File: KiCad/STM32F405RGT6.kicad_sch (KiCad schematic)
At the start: 53 parts, among them J1 Conn_02x05_Odd_Even, J2 USB_C_Receptacle_USB2.0, SW1 TS-1187A, SW2 TS-1187A, U1 M24C02-RMN, U2 STM32F405RGTx, U3 AMS1117-3.3, U4 SRV05-4, Y1 16MHz

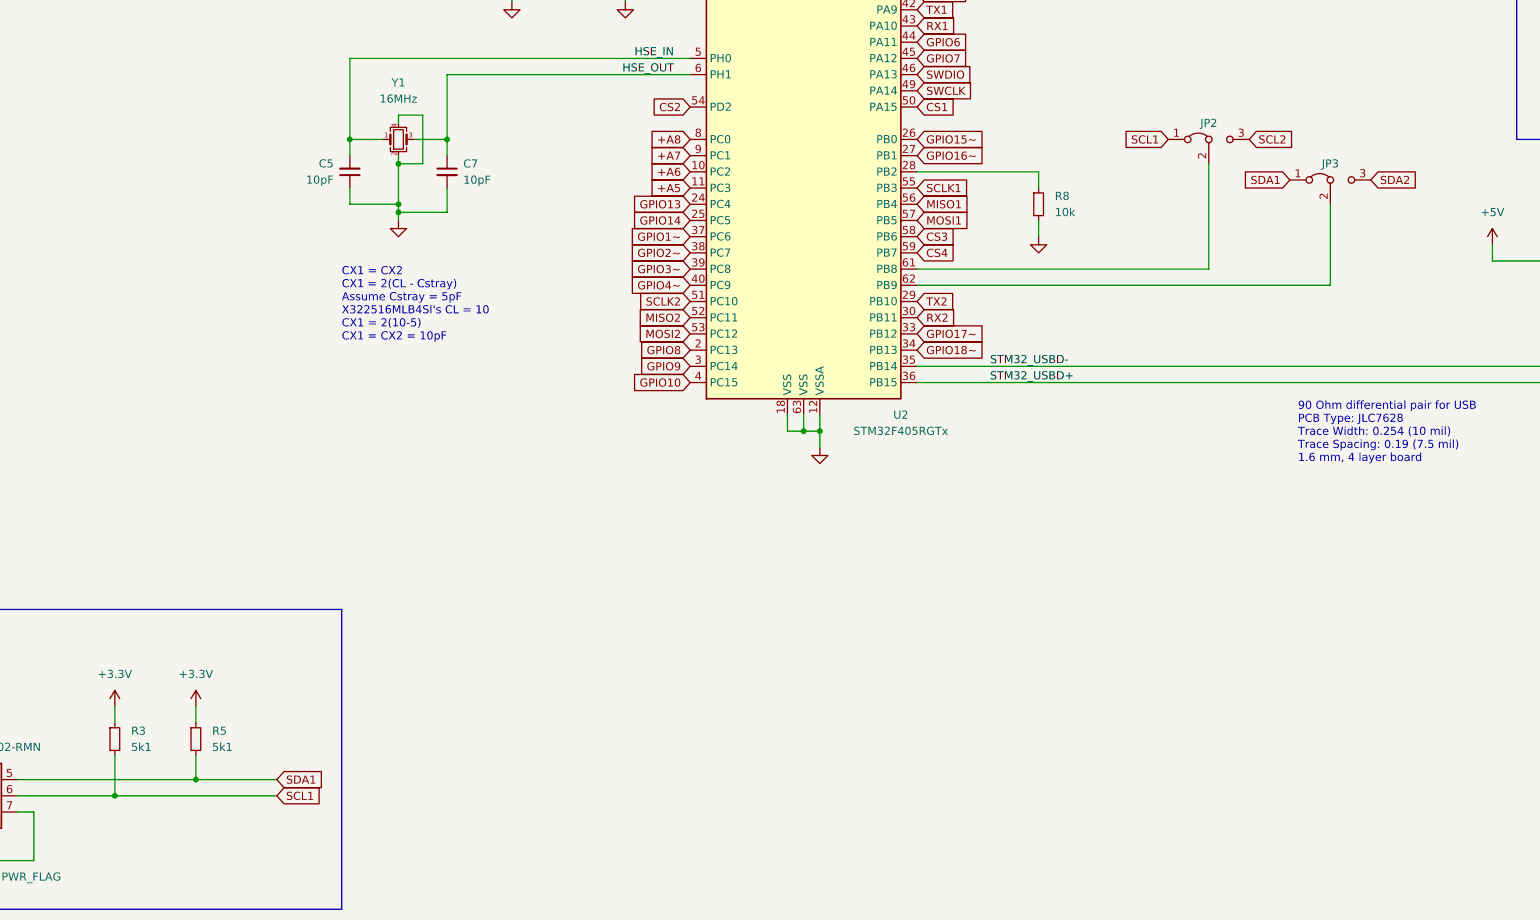
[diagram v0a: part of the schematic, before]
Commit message: Updated PCB and Schematic
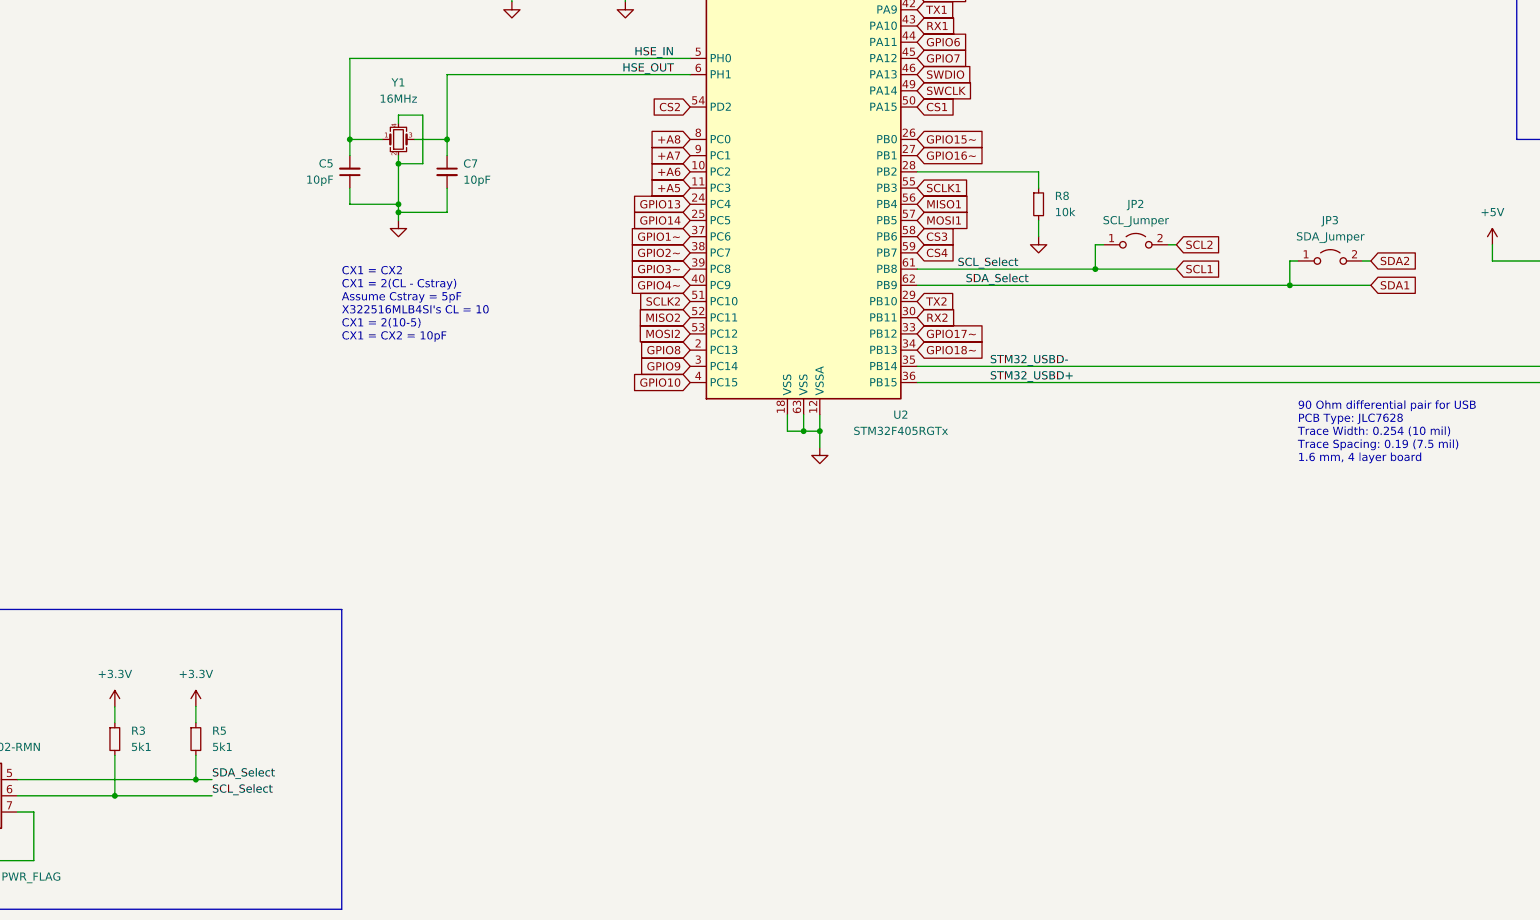
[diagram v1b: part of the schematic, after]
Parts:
- removed JP2, JP3: SDA_Jumper, Jumper:SolderJumper-3_P1.3mm_Bridged12_RoundedPad1.0x1.5mm, symbol Jumper:Jumper_3_Bridged12
- added JP2: SCL_Jumper, Jumper:SolderJumper-2_P1.3mm_Open_RoundedPad1.0x1.5mm, symbol Jumper:Jumper_2_Open
- added JP3: SDA_Jumper, Jumper:SolderJumper-2_P1.3mm_Open_RoundedPad1.0x1.5mm, symbol Jumper:Jumper_2_Open
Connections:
- net SCL1: now also U2.61 (PB8), JP2.1 (A)
- net SCL2: now also JP2.2 (B)
- net SDA1: now also U2.62 (PB9), JP3.1 (A)
- net SDA2: now also JP3.2 (B)
